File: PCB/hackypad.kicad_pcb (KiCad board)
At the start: 2 copper layers, 87 x 80 mm, 26 parts, among them SW1 SW_Push_45deg, SW10 RotaryEncoder_Switch, SW2 SW_Push_45deg, SW3 SW_Push_45deg, SW4 SW_Push_45deg, SW5 SW_Push_45deg, SW6 SW_Push_45deg, SW7 SW_Push_45deg, SW8 SW_Push_45deg, SW9 SW_Push_45deg, U1 MOUDLE-SEEEDUINO-XIAO, U2 ER_OLEDM0.91_1x-I2C

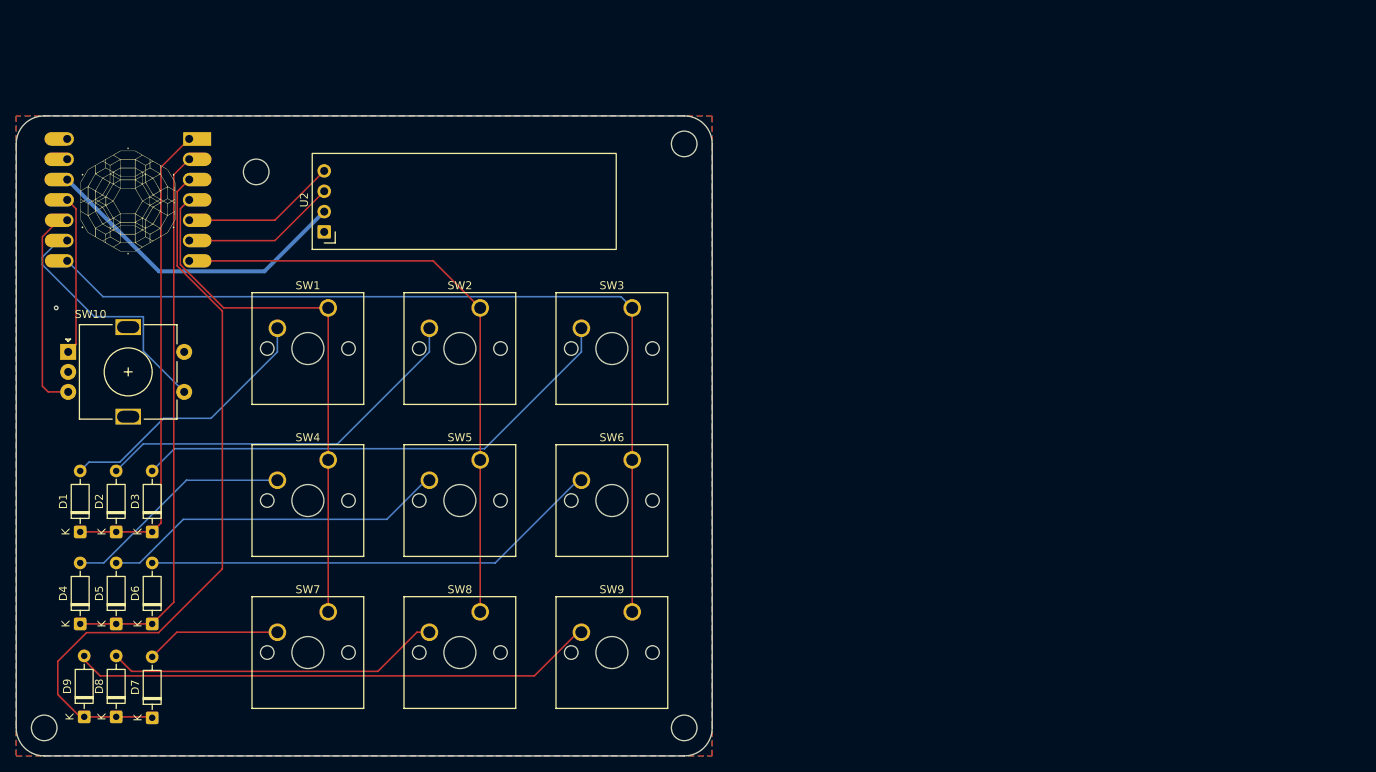
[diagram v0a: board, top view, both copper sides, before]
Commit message: feat(PCB): Rework the pcb
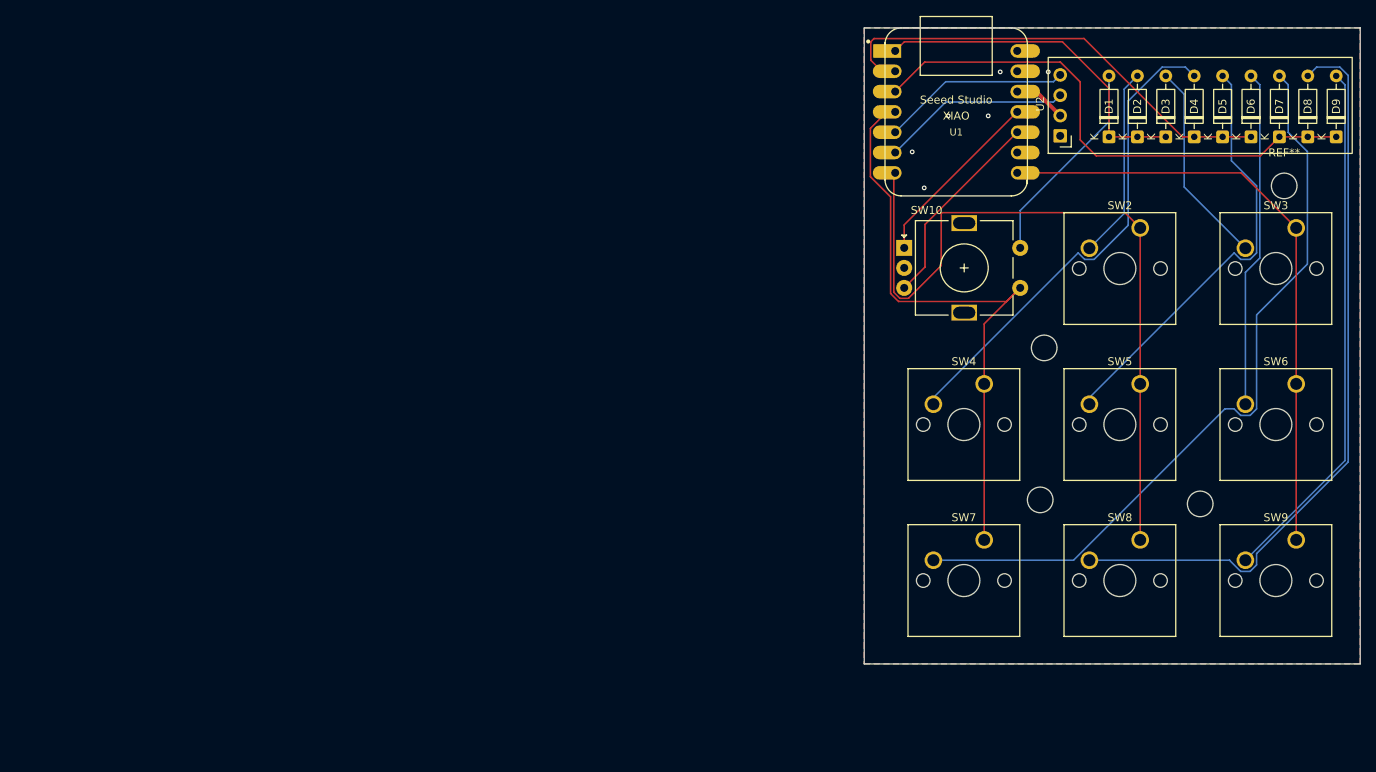
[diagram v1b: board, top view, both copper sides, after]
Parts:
- removed G***: LOGO, LOGO
- removed the REF** at (95.5, 55.5)
- removed the REF** at (149.0, 125.0)
- removed the REF** at (149.0, 52.0)
- removed the REF** at (69.0, 125.0)
- removed SW1: SW_Push_45deg, switch:SW_Cherry_MX_1.00u_PCB
- added REF**: MountingHole_3.2mm_M3, MountingHole:MountingHole_3.2mm_M3, F.Cu at (224.0, 57.2)
- added REF**: MountingHole_3.2mm_M3, MountingHole:MountingHole_3.2mm_M3, F.Cu at (213.5, 97.0)
- added REF**: MountingHole_3.2mm_M3, MountingHole:MountingHole_3.2mm_M3, F.Cu at (193.5, 96.5)
- added REF**: MountingHole_3.2mm_M3, MountingHole:MountingHole_3.2mm_M3, F.Cu at (194.0, 77.5)
- U1: moved to F.Cu
- moved D9 172.5 mm to (230.5, 51.1)
- moved D8 165.7 mm to (226.9, 51.1)
- moved D7 158.5 mm to (223.4, 51.1)
- moved D4 152.0 mm to (212.8, 51.1)
- moved D5 151.1 mm to (216.3, 51.1)
- moved D6 150.2 mm to (219.8, 51.1)
- moved D1 137.8 mm to (202.1, 51.1)
- moved D2 136.9 mm to (205.7, 51.1)
- moved D3 136.0 mm to (209.2, 51.1)
- moved SW10 105.3 mm to (176.5, 65.0)
- moved U1 104.1 mm to (183.0, 48.0), turned to 0 degrees
- moved U2 92.8 mm to (196.0, 51.0)
- moved SW3 83.6 mm to (225.5, 62.5)
- moved SW6 83.5 mm to (225.5, 82.0)
- moved SW9 83.5 mm to (225.5, 101.5)
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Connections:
- D1 pad 2: Net-(D1-A) -> Encoder S2
- SW10 pad S1: Encoder Sw -> Col 0
- SW10 pad S2: GND -> Encoder S2
- U1 pad 9: Encoder Sw -> unconnected-(U1-PA7_A8_D8_SCK-Pad9)
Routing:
- net Net-(D7-A): track 16.9 -> 94.6 mm
- net Net-(D8-A): track 42.0 -> 93.7 mm
- net Net-(D3-A): track 62.8 -> 25.7 mm
- net Col 2: track 111.1 -> 76.7 mm
- net Net-(D1-A): track 33.8 -> 0.00 mm
- net VCC: track 40.0 -> 6.62 mm
- net Net-(D4-A): track 28.9 -> 60.8 mm
- net Encoder Sw: track 31.7 -> 0.00 mm
- net Row 2: track 94.1 -> 66.7 mm
- net Encoder S2: track 0.00 -> 26.1 mm
- net Net-(D2-A): track 48.3 -> 24.0 mm
- net Col 1: track 76.8 -> 94.2 mm
- net Row 0: track 60.0 -> 42.8 mm
- net Net-(D6-A): track 57.9 -> 42.2 mm
- net Net-(D5-A): track 43.4 -> 53.8 mm
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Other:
- board size 87 x 80 mm -> 62 x 79.5 mm
